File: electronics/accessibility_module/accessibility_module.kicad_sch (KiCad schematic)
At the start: 11 parts, among them J1 Conn_01x05_Pin, M1 Motor_DC, M2 SG90, M3 SG90, M4 SG90, M5 SG90, Q1 BC546, U1 ESP32_DevKit_V1_DOIT, U2 LM1117T-3.3

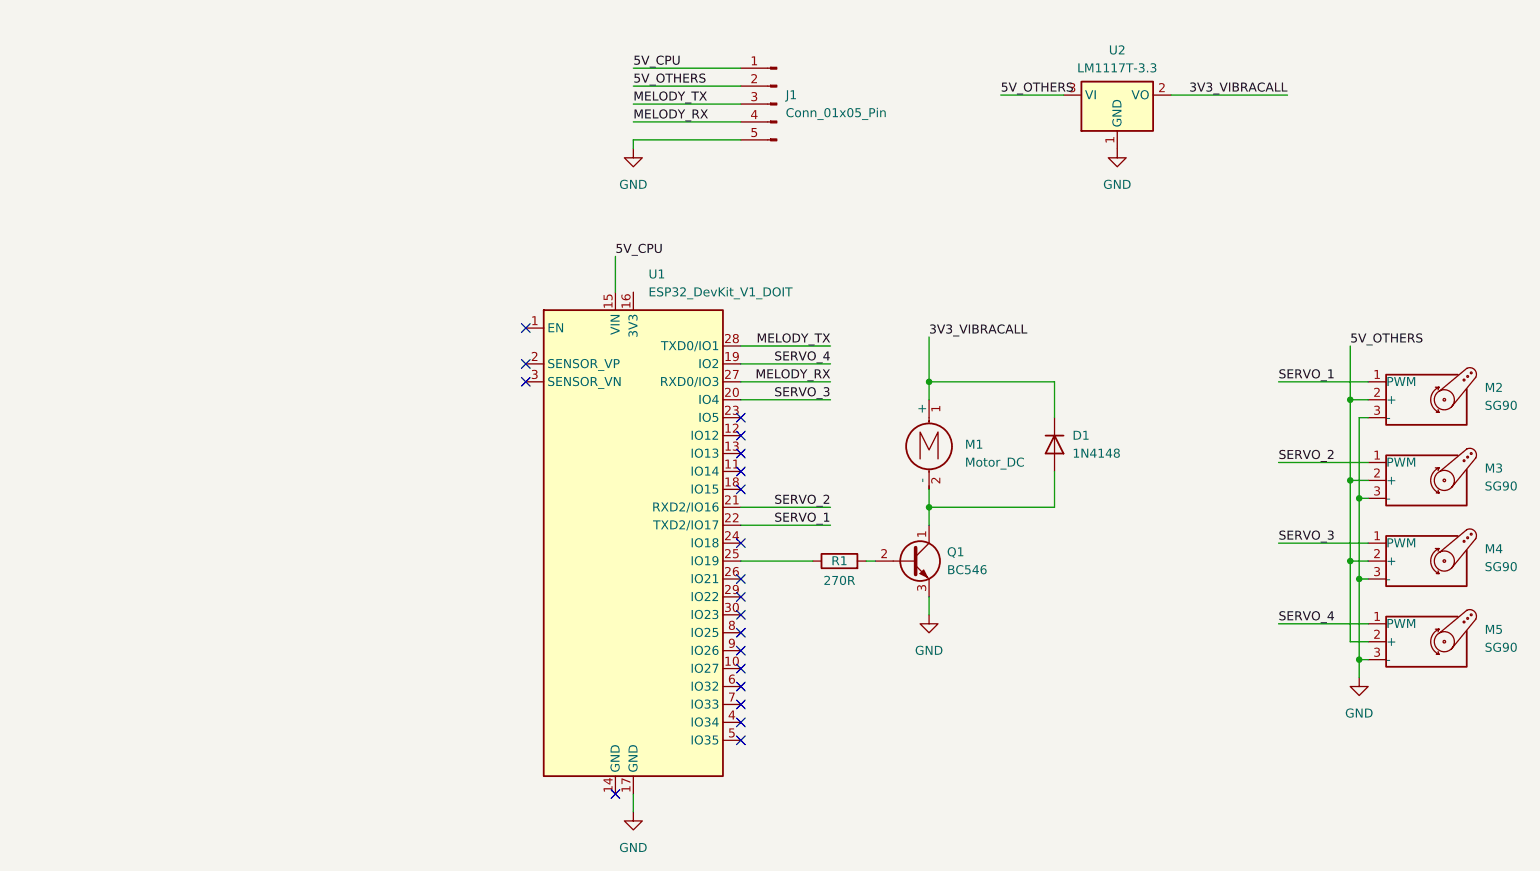
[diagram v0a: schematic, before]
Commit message: Atualização esquemático eletrônico
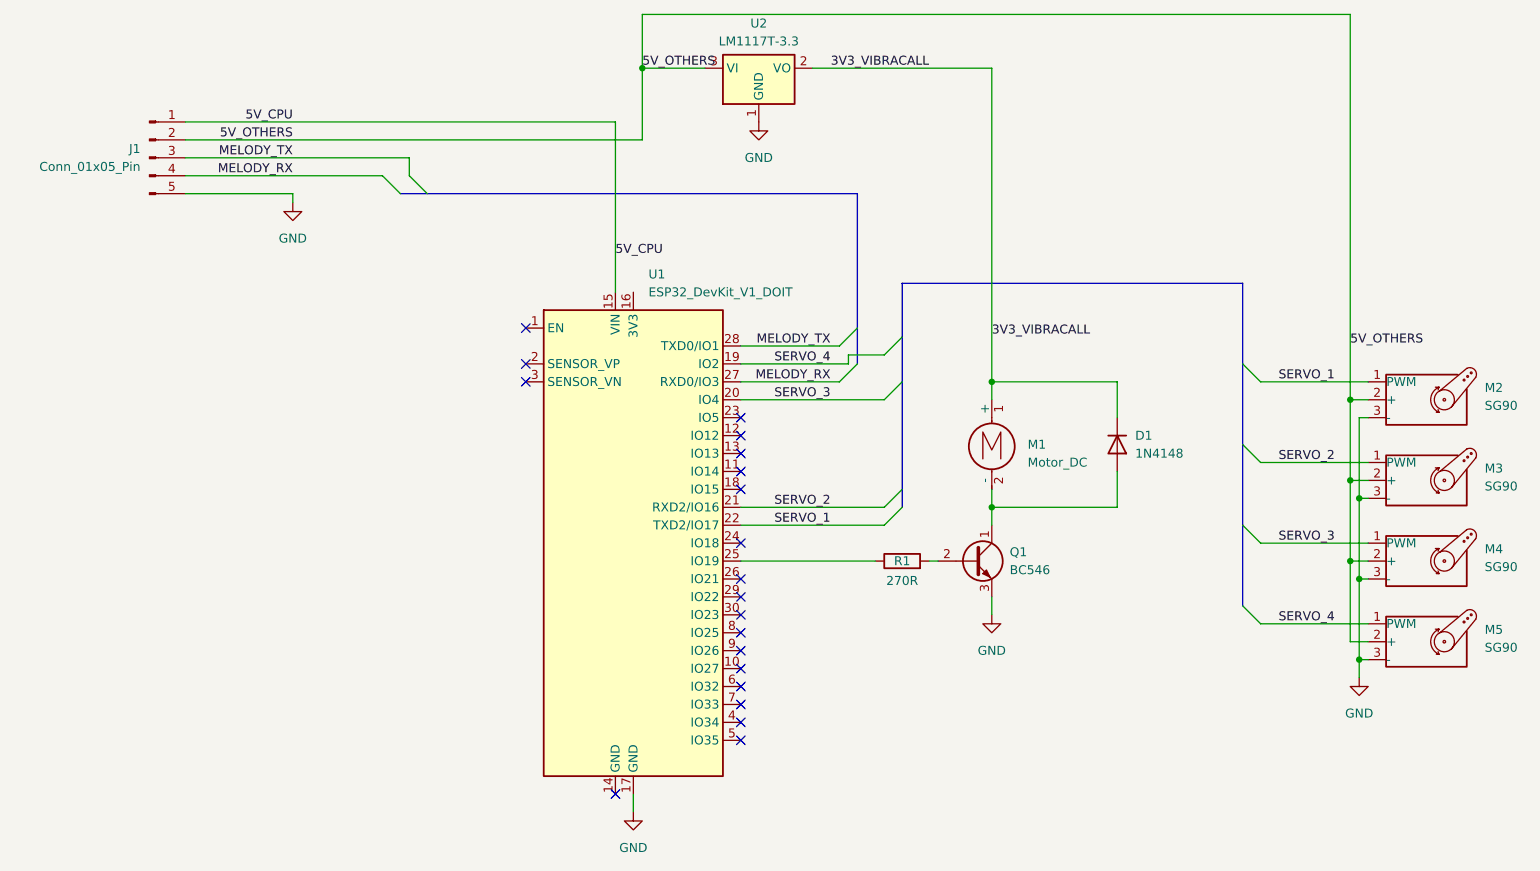
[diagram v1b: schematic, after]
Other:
- moved on the sheet: D1, J1, M1, Q1, R1, U2
